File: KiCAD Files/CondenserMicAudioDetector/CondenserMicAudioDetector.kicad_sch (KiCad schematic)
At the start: 29 parts, among them Q1 BC547, Q2 BC547, Q3 BC547, Q4 BC557

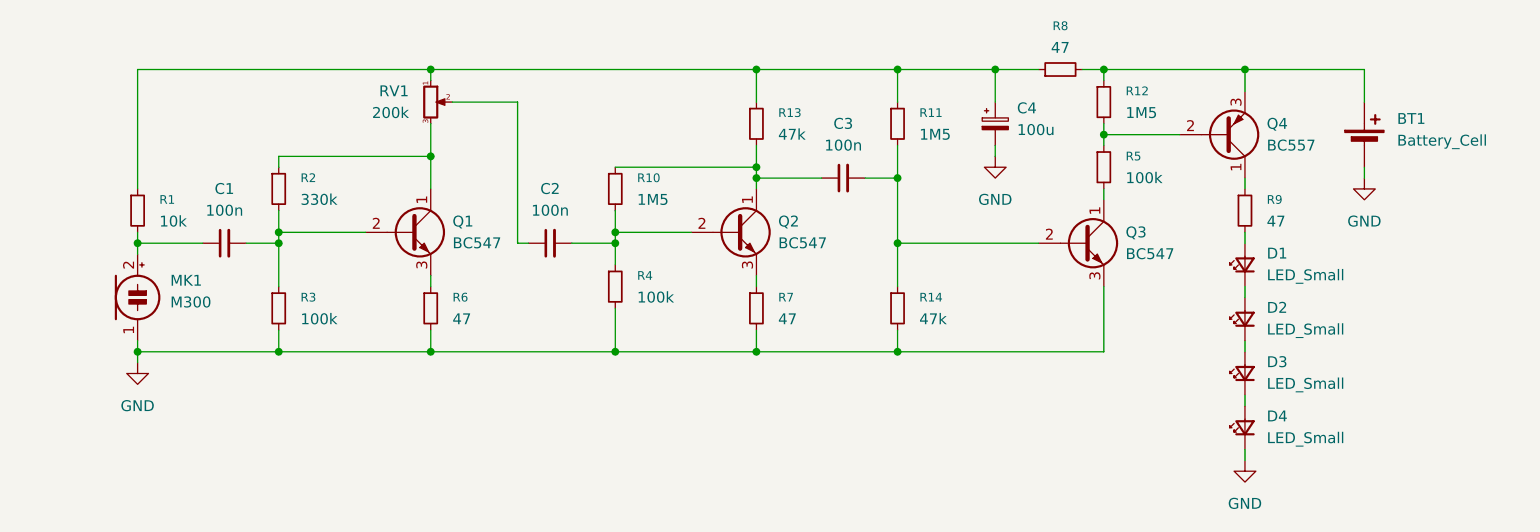
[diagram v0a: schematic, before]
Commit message: Updated Schematic & PCB Design
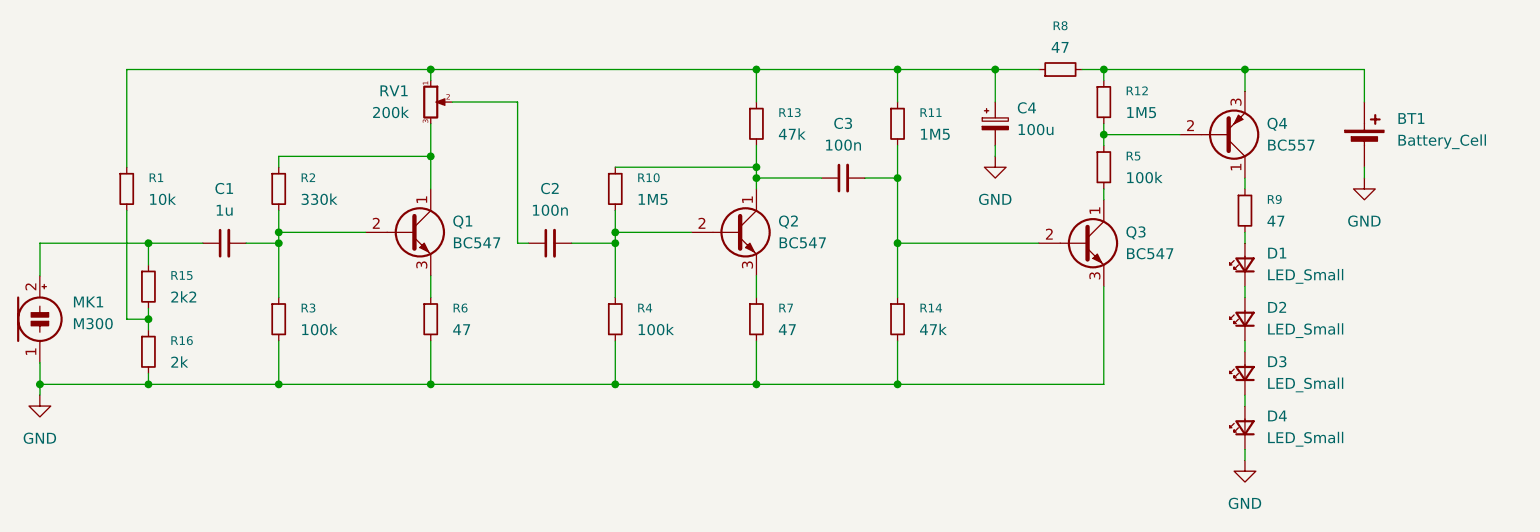
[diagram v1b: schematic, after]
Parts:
- added R15: 2k2, Resistor_SMD:R_0805_2012Metric_Pad1.20x1.40mm_HandSolder, symbol Device:R_Small
- added R16: 2k, Resistor_SMD:R_0805_2012Metric_Pad1.20x1.40mm_HandSolder, symbol Device:R_Small
- C1: value 100n -> 1u
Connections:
- net GND: now also R16.2
- net at C1.1, MK1.2 (+): now also R15.1; no longer R1.2
- new net: R1.2, R15.2, R16.1
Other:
- moved on the sheet: MK1, R1, R14, R3, R4, R6, R7
